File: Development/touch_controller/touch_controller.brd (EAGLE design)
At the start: 50 x 50 mm, 44 parts, among them IC1 LPC812M101JDH16, IC2 CY8C201A0-SX2I, IC3 BMA250E, SW1 SK-12D01-VG4, U1 RN4020-V/RM123

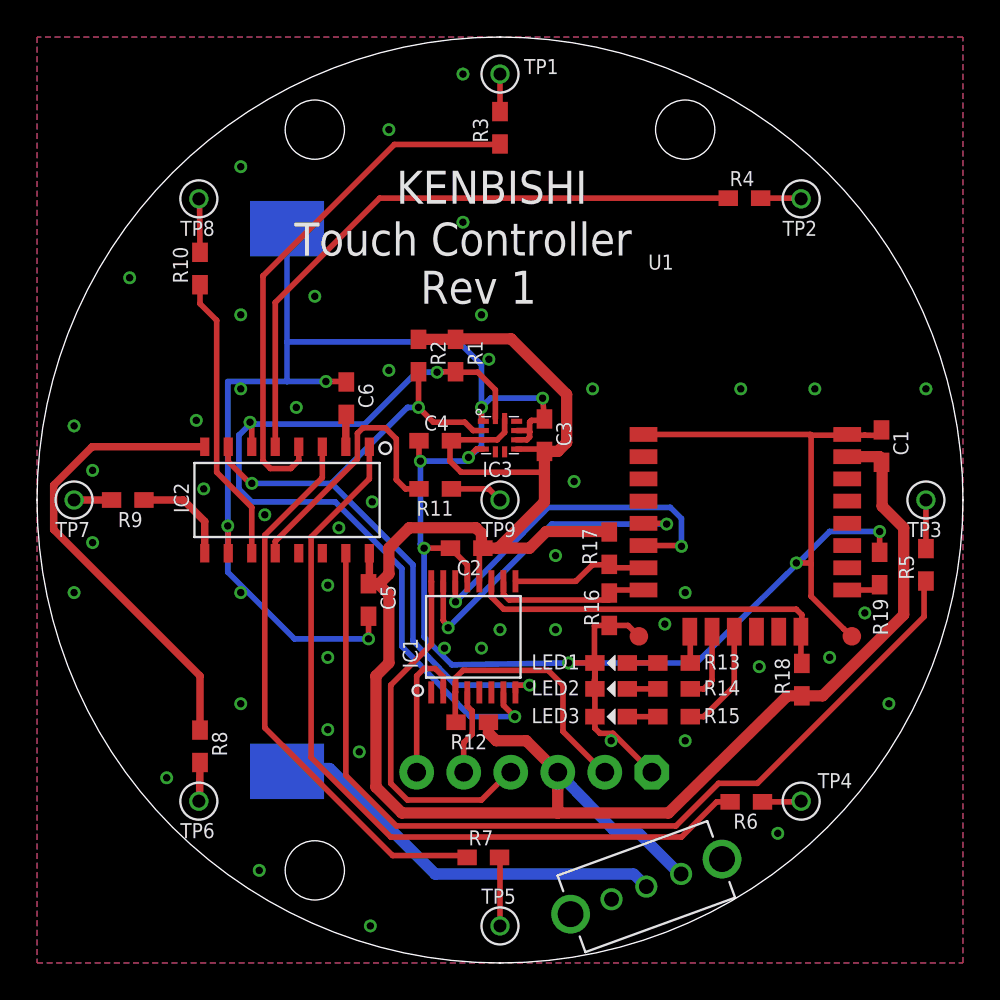
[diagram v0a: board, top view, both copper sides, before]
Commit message: touch_controller rev2
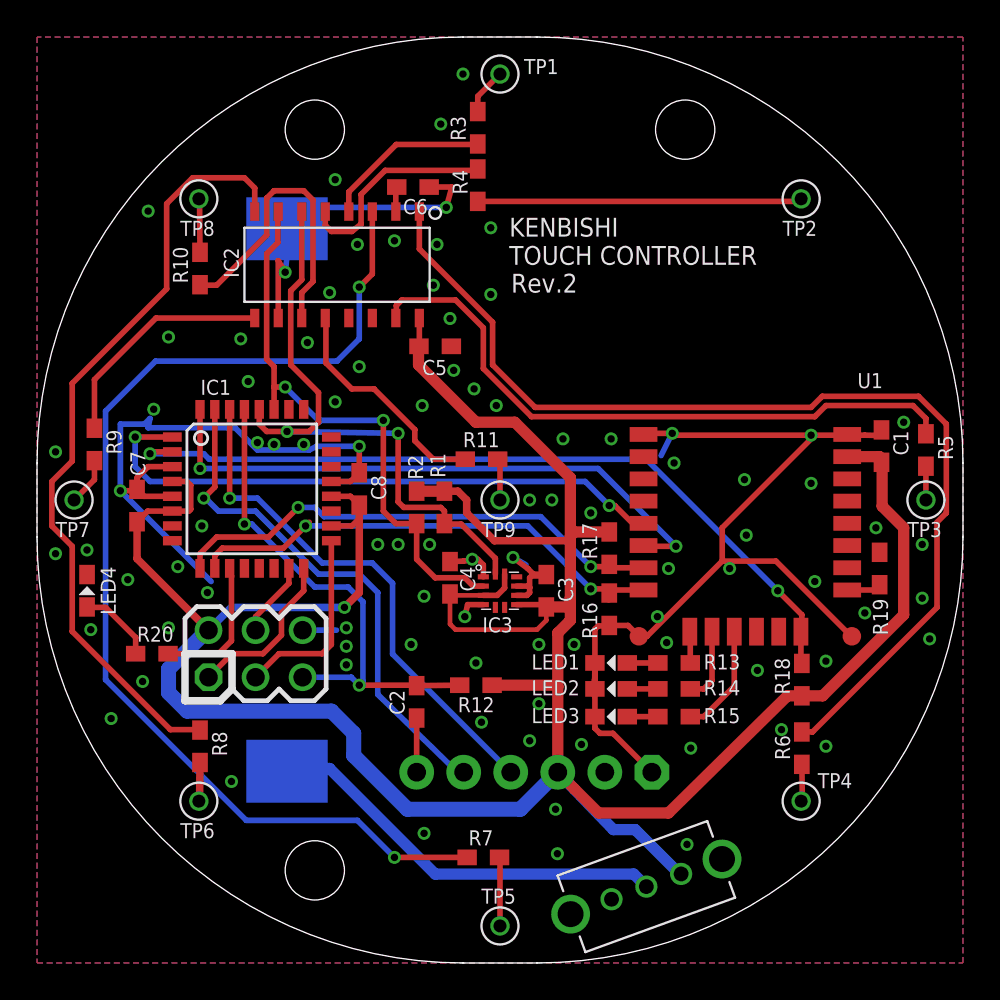
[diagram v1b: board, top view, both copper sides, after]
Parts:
- added C7, C8: 0.1u, generic:SMD1608_REDUCED
- added LED4: (no value), generic:LED1608_REDUCED
- added R20: 1k, generic:SMD1608_REDUCED
- added U$1: M03X2STD, header:2X03
- IC1: value LPC812M101JDH16 -> ATMEGA328P-AU; device micro_controller:TSSOP16 -> AVR:TQFP32-08
- moved R4 14.4 mm to (23.8, 42.0), turned to 270 degrees
- moved IC1 14.4 mm to (11.6, 25.6)
- moved C5 14.2 mm to (21.5, 33.3), turned to 0 degrees
- moved IC2 13.0 mm to (16.2, 37.7)
- moved C6 12.0 mm to (20.3, 41.9), turned to 180 degrees
- moved C2 8.73 mm to (20.5, 14.1), turned to 90 degrees
- moved C3 8.40 mm to (27.5, 20.1)
- moved IC3 8.40 mm to (25.0, 20.1)
- moved R1 8.22 mm to (22.0, 24.6)
- moved R2 8.20 mm to (20.5, 24.6)
- moved C4 7.44 mm to (22.3, 20.8), turned to 90 degrees
- moved R5 6.20 mm to (48.0, 27.7), turned to 270 degrees
- moved R6 4.17 mm to (41.3, 11.6), turned to 270 degrees
- moved R9 3.50 mm to (3.10, 28.0), turned to 270 degrees
- moved R11 2.97 mm to (24.0, 27.2)
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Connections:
- removed net ISP_EN: IC1.2, JP1.6
- removed net ISP_RXD: IC1.16, JP1.4
- removed net ISP_TXD: IC1.4, JP1.5
- new net MISO: IC1.16, U$1.1
- new net MOSI: IC1.15, U$1.4
- new net N$13: IC1.11, R20.2
- new net N$17: LED4.A, R20.1
- new net RESET: C2.1, JP1.6
- new net RXD: IC1.30, JP1.4
- new net SCK: IC1.17, U$1.3
- new net TXD: IC1.31, JP1.5
- net +3V3: now also C7.2, C8.2, IC1.18, IC1.20, IC1.4, IC1.6, U$1.2; no longer C2.1, IC1.12
- net BLE_RX: now also IC1.32; no longer IC1.14
- net BLE_TX: now also IC1.1; no longer IC1.15
- net GND: now also C7.1, C8.1, IC1.21, IC1.3, IC1.5, LED4.K, U$1.6; no longer C2.2, IC1.13
- net RST: now also C2.2, IC1.29, U$1.5; no longer IC1.3, JP1.2
- net SCL: now also IC1.28; no longer IC1.7
- net SDA: now also IC1.27; no longer IC1.8
- net WAKE_HW: now also IC1.2; no longer IC1.11
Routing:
- net +3V3: track 124.3 -> 165.1 mm, vias 0 -> 1
- net GND: track 152.5 -> 118.9 mm, vias 60 -> 91
- net GP0_4: track 30.3 -> 60.5 mm, vias 0 -> 2
- net TXD: track 0.00 -> 28.5 mm, vias 0 -> 1
- net RXD: track 0.00 -> 28.4 mm, vias 0 -> 1
- net GP0_1: track 34.6 -> 11.4 mm
- net WAKE_HW: track 20.7 -> 42.7 mm, vias 0 -> 2
- net WAKE_SW: track 7.54 -> 27.3 mm, vias 0 -> 2
- net GP0_0: track 28.8 -> 9.09 mm
- net ISP_RXD: track 19.3 -> 0.00 mm
- net CMD/MLDP: track 8.81 -> 26.7 mm, vias 0 -> 2
- net GP0_2: track 51.3 -> 34.7 mm
- net GP1_0: track 25.5 -> 42.1 mm
- net N$4: track 2.20 -> 17.6 mm
- net BLE_TX: track 18.0 -> 32.4 mm
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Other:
- outline, holes or cut-outs redrawn
- board text added: "KENBISHI TOUCH CONTROLLER"
- board text added: "Rev.2"
- board text removed: "KENBISHI"
- board text removed: "Rev 1"
- board text removed: "Touch Controller"
